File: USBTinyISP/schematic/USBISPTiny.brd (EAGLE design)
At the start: 83 x 30 mm, 57 parts, among them Q1 12MHz, T1 BC847, T10 BC847, T2 BC847, T3 BC847, T4 BC847, T5 BC847, T6 BC847, T9 BC847, X1 USB_B, X2 Target_MCU

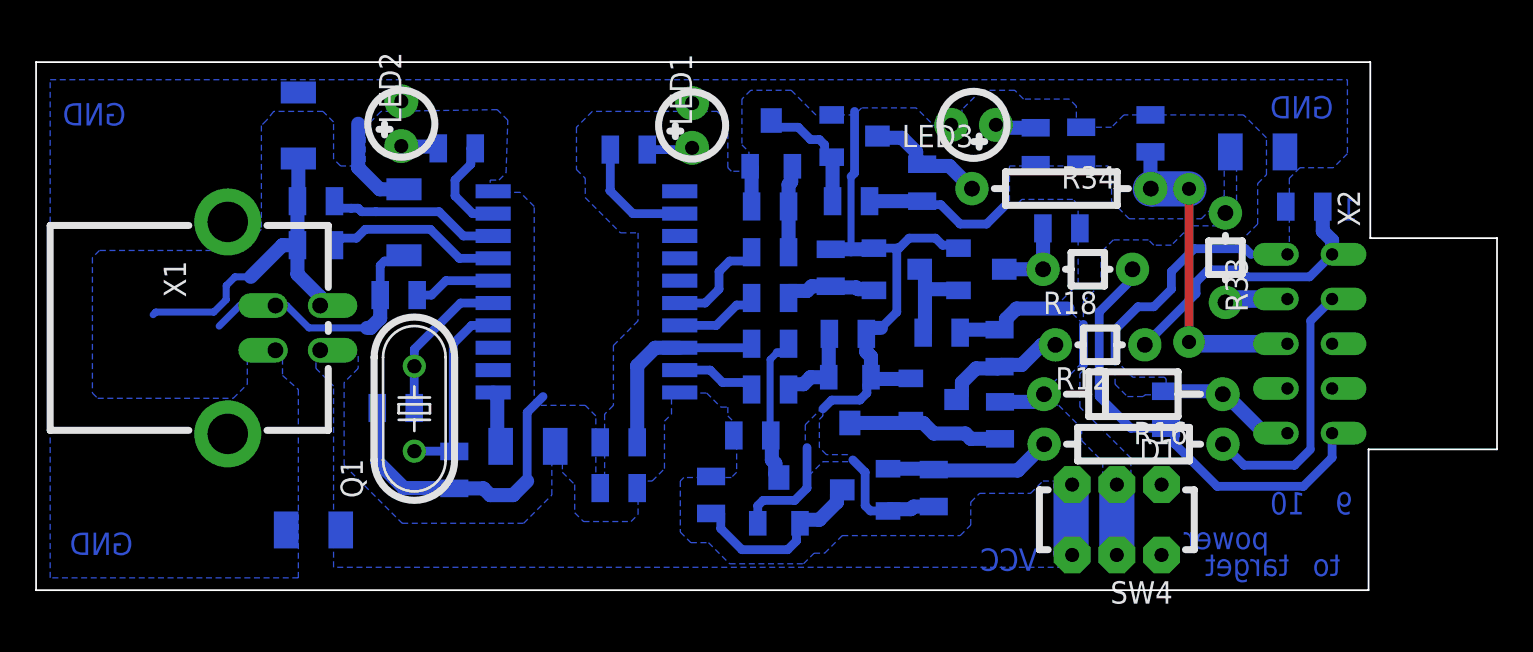
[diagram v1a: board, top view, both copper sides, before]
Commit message: TinyISP. Fix micro usb incorrect pinout. Change transystor levels converter to fast, diode based. Route PCB.
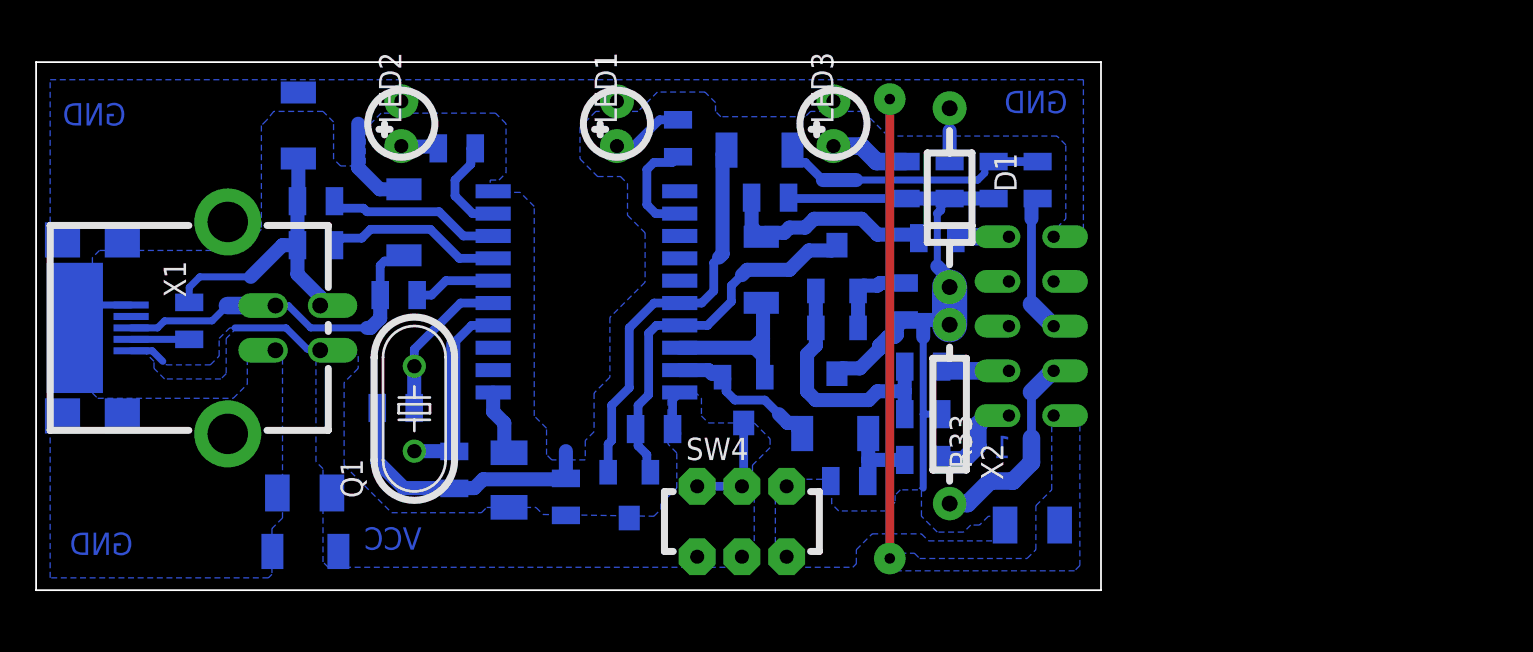
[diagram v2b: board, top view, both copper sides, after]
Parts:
- removed C11, C18, C7, C9: 100pF, __MyCommonLib1:RSMD_0805
- removed R13, R14, R15, R19, R20, R26, R35, R36, R9: 4K7, __MyCommonLib1:RSMD_0805
- removed R16: 4K7, __MyCommonLib1:R0207
- removed R28: 1K0, __MyCommonLib1:RSMD_0805
- removed R30: 100R, __MyCommonLib1:RSMD_0805
- removed T1, T10, T2, T3, T4, T5, T9: BC847, __MyCommonLib1:SOT23_SMALL_PADS
- added D10, D2, D3: LL4148, __MyCommonLib1:SOD-80
- added DD4, DD5, DD6: BAT54C, __MyCommonLib1:SOT23_SMALL_PADS
- added J10: 0, __MyCommonLib1:RSMD_0805
- added R7: 100R, __MyCommonLib1:RSMD_0805
- added R8: 4K7, __MyCommonLib1:RSMD_0805
- added X3: USB_MICRO, __MyCommonLib1:USB_MICRO_TYPE_B
- added ZD3: 5.6V, __MyCommonLib1:SOD-80
- R12, R18: device __MyCommonLib1:R0204 -> __MyCommonLib1:RSMD_0805
- R27: value 4K7 -> 1K0
- R33: device __MyCommonLib1:R0204 -> __MyCommonLib1:R0207
- R34: device __MyCommonLib1:R0207 -> __MyCommonLib1:RSMD_0805
- moved C3 24.8 mm to (56.6, 3.70)
- moved SW4 21.3 mm to (40.1, 3.90), turned to 0 degrees
- moved X2 20.9 mm to (54.0, 15.0), turned to 270 degrees
- moved R33 18.0 mm to (51.9, 10.0)
- moved R17 16.6 mm to (41.7, 22.3)
- moved D1 15.3 mm to (51.9, 22.3), turned to 270 degrees
- moved T6 12.7 mm to (45.5, 18.3), turned to 180 degrees
- moved R12 12.0 mm to (50.4, 7.40), flipped to the bottom, turned to 180 degrees
- moved R10 11.4 mm to (46.2, 6.20), turned to 180 degrees
- moved R18 8.73 mm to (51.2, 20.0), flipped to the bottom, turned to 180 degrees
- moved LED3 7.96 mm to (45.3, 26.5), turned to 90 degrees
- moved C16 7.73 mm to (51.9, 23.3)
- moved R31 7.64 mm to (49.4, 23.3)
- moved R27 4.95 mm to (35.1, 9.15), turned to 0 degrees
- moved LED1 4.27 mm to (33.0, 26.5)
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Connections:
- removed net N$20: R17.PAD_1, R18.PAD_0, T3.3
- removed net N$22: R15.PAD_1, T3.1, T4.3
- removed net N$23: R11.PAD_1, R16.PAD_0, T6.1
- removed net N$24: R19.PAD_1, R20.PAD_0, T4.1
- removed net N$33: R28.PAD_1, R30.PAD_0, T5.3
- removed net N$35: R27.PAD_1, T5.1, T6.3
- removed net N$40: R26.PAD_1, T10.3, T9.1
- removed net N$41: R35.PAD_1, R36.PAD_0, T10.1
- new net N$10: J10.PAD_1, X3.2
- new net N$13: D10.ANODE, R17.PAD_1, R18.PAD_0
- net +5V_USB: now also DD4.3, DD5.3, SW4.CENTER1, SW4.CENTER2, SW4.POS_A1, SW4.POS_A2, X3.1, ZD3.CATHODE; no longer R28.PAD_0, SW4.POS_B1, SW4.POS_B2
- net GND: now also X3.5, X3.PACKAGE1, X3.PACKAGE2, X3.PACKAGE3, X3.PACKAGE4, X3.PACKAGE5, ZD3.ANODE; no longer C11.PAD_0, C18.PAD_0, C7.PAD_0, C9.PAD_0, R11.PAD_0, R13.PAD_0, R19.PAD_0, R35.PAD_0, T1.2, T10.2, T2.2, T3.2, T4.2, T5.2, T6.2, T9.2
- net N$11: now also DD6.2, R8.PAD_0, T6.1; no longer R13.PAD_1, R14.PAD_0, T2.1
- net N$2: now also D3.ANODE; no longer T1.3
- net N$39: now also D2.ANODE; no longer T9.3
- net N$9: now also DD6.1, R11.PAD_0, R7.PAD_0, T6.2; no longer R9.PAD_1, T1.1, T2.3
- net SPI_MISO: now also DD4.2, R27.PAD_1, T6.3, U$1.17; no longer C11.PAD_1, R30.PAD_1, U$1.18
- net SPI_MOSI: now also D10.CATHODE, DD5.2, U$1.18; no longer R20.PAD_1, U$1.17
- net SPI_RST: now also D2.CATHODE, DD4.1; no longer R36.PAD_1
- net SPI_SCK: now also D3.CATHODE, DD5.1; no longer R14.PAD_1
- net T_MISO: now also R7.PAD_1; no longer R16.PAD1
- net T_MOSI: now also R18.PAD_1; no longer C9.PAD_1, R18.PAD1
- net T_RST: now also R34.PAD_1; no longer C18.PAD_1, R34.PAD1
- net T_SCK: now also R12.PAD_1; no longer C7.PAD_1, R12.PAD1
- net T_VCC: now also DD6.3, R11.PAD_1, R8.PAD_1, SW4.POS_B1, SW4.POS_B2; no longer R15.PAD_0, R26.PAD_0, R9.PAD_0, SW4.CENTER1, SW4.CENTER2
- net USB_D+: now also X3.3
- net USB_D-: now also J10.PAD_0
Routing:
- net GND: track 91.3 -> 53.8 mm, vias 0 -> 2
- net T_MOSI: track 25.7 -> 3.05 mm
- net SPI_RST: track 6.16 -> 22.7 mm
- net T_VCC: track 24.6 -> 38.5 mm
- net N$13: track 0.00 -> 12.3 mm
- net +5V_USB: track 4.11 -> 16.2 mm
- net T_MISO: track 14.9 -> 3.92 mm
- net N$35: track 10.9 -> 0.00 mm
- net T_SCK: track 16.4 -> 5.57 mm
- net T_RST: track 18.7 -> 8.13 mm, vias 2 -> 0
- net SPI_MISO: track 11.5 -> 21.9 mm
- net N$23: track 9.53 -> 0.00 mm
- net N$39: track 6.82 -> 15.8 mm
- net N$33: track 8.62 -> 0.00 mm
- net N$25: track 3.60 -> 11.4 mm
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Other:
- board size 83 x 30 mm -> 60.5 x 30 mm
- board text removed: "10"
- board text removed: "9"
- board text removed: "power"
- board text removed: "target"
- board text removed: "to"
